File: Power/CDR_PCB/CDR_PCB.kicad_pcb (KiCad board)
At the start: 2 copper layers, 161.5 x 80 mm, 0 parts

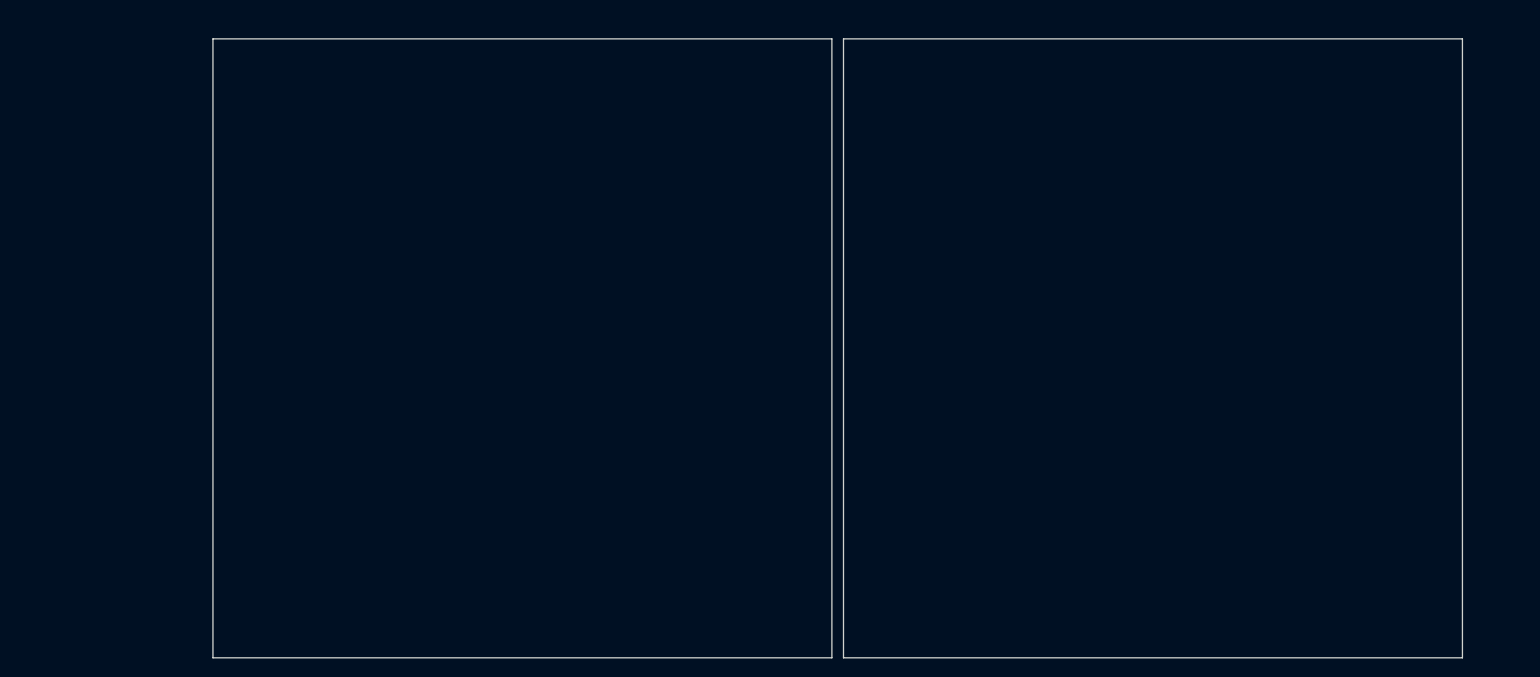
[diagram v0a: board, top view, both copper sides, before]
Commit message: Updated PCB
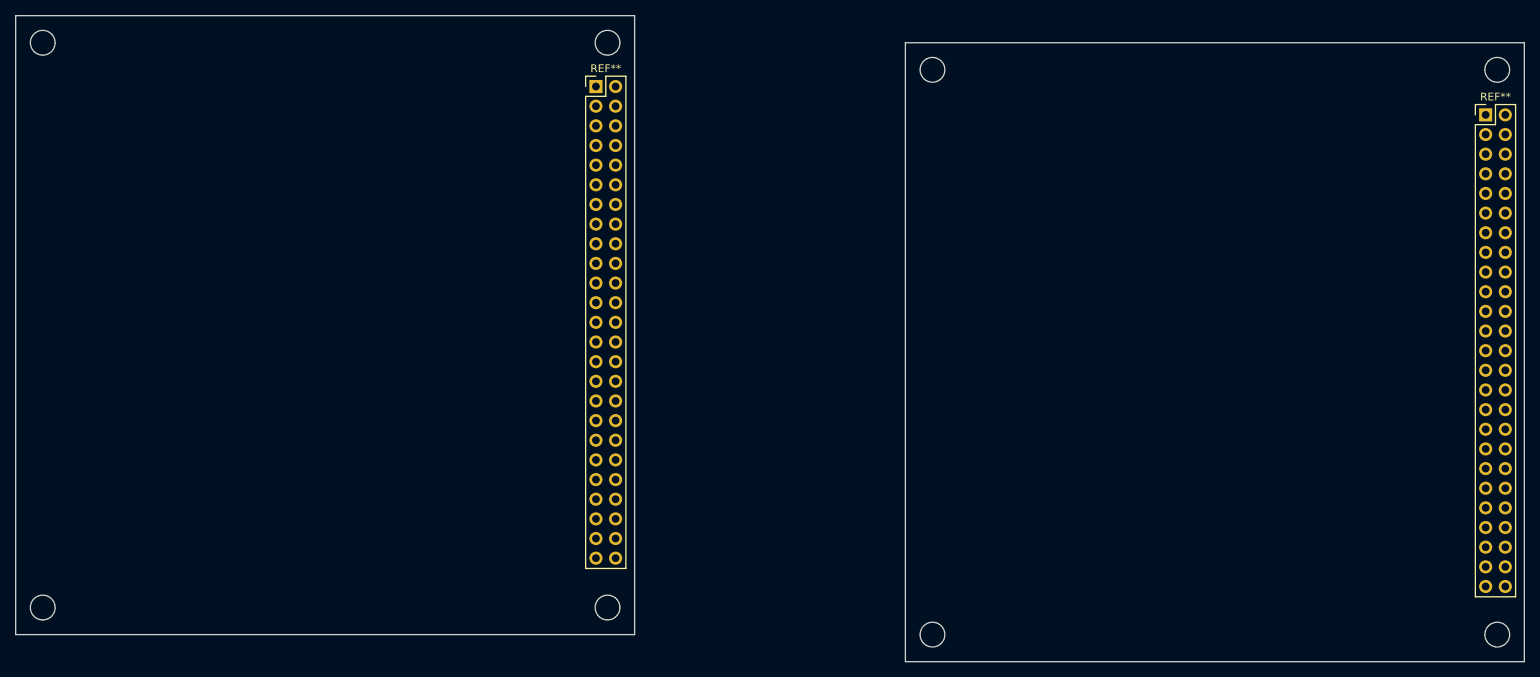
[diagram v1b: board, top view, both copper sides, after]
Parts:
- added REF**: MountingHole_3.2mm_M3, MountingHole:MountingHole_3.2mm_M3, F.Cu at (140.0, 112.5)
- added REF**: MountingHole_3.2mm_M3, MountingHole:MountingHole_3.2mm_M3, F.Cu at (255.0, 43.0)
- added REF**: MountingHole_3.2mm_M3, MountingHole:MountingHole_3.2mm_M3, F.Cu at (255.0, 116.0)
- added REF**: PinHeader_2x25_P2.54mm_Vertical, Connector_PinHeader_2.54mm:PinHeader_2x25_P2.54mm_Vertical, F.Cu at (138.5, 45.2)
- added REF**: MountingHole_3.2mm_M3, MountingHole:MountingHole_3.2mm_M3, F.Cu at (182.0, 43.0)
- added REF**: MountingHole_3.2mm_M3, MountingHole:MountingHole_3.2mm_M3, F.Cu at (67.0, 39.5)
- added REF**: MountingHole_3.2mm_M3, MountingHole:MountingHole_3.2mm_M3, F.Cu at (67.0, 112.5)
- added REF**: MountingHole_3.2mm_M3, MountingHole:MountingHole_3.2mm_M3, F.Cu at (140.0, 39.5)
- added REF**: MountingHole_3.2mm_M3, MountingHole:MountingHole_3.2mm_M3, F.Cu at (182.0, 116.0)
- added REF**: PinHeader_2x25_P2.54mm_Vertical, Connector_PinHeader_2.54mm:PinHeader_2x25_P2.54mm_Vertical, F.Cu at (253.5, 48.8)
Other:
- board size 161.5 x 80 mm -> 195 x 83.5 mm
